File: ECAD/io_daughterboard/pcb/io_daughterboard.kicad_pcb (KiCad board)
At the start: 2 copper layers, 120 x 66 mm, 90 parts, among them CON1 BARREL_JACK, J1 XF2L-0625-1A, J2 FH12A-40S-0.5SH, P1 CONN_02X32, P10 Slave 5B, P11 Slave 1C, P12 Slave 3C, P13 Slave 4C, P14 Slave 5C, P15 Slave 1D, P16 Slave 3D, P17 Slave 4D, P18 Slave 5D, P19 MIDI, P2 CONN_02X32, P3 Slave 1A, P4 Slave 3A, P5 Slave 4A, P6 Slave 5A, P7 Slave 1B, P8 Slave 3B, P9 Slave 4B, SW1 Reset, SW2 User, U1 FAN5333BSX, U10 SN74LV1T34DCKR, U11 SN74LV1T34DCKR, U2 SPX3819M5-L-3-3, U3 74HC244, U4 74HC244, U5 74HC244, U6 STMPE811QTR, U7 74HC244, U8 74HC244, U9 74HC244

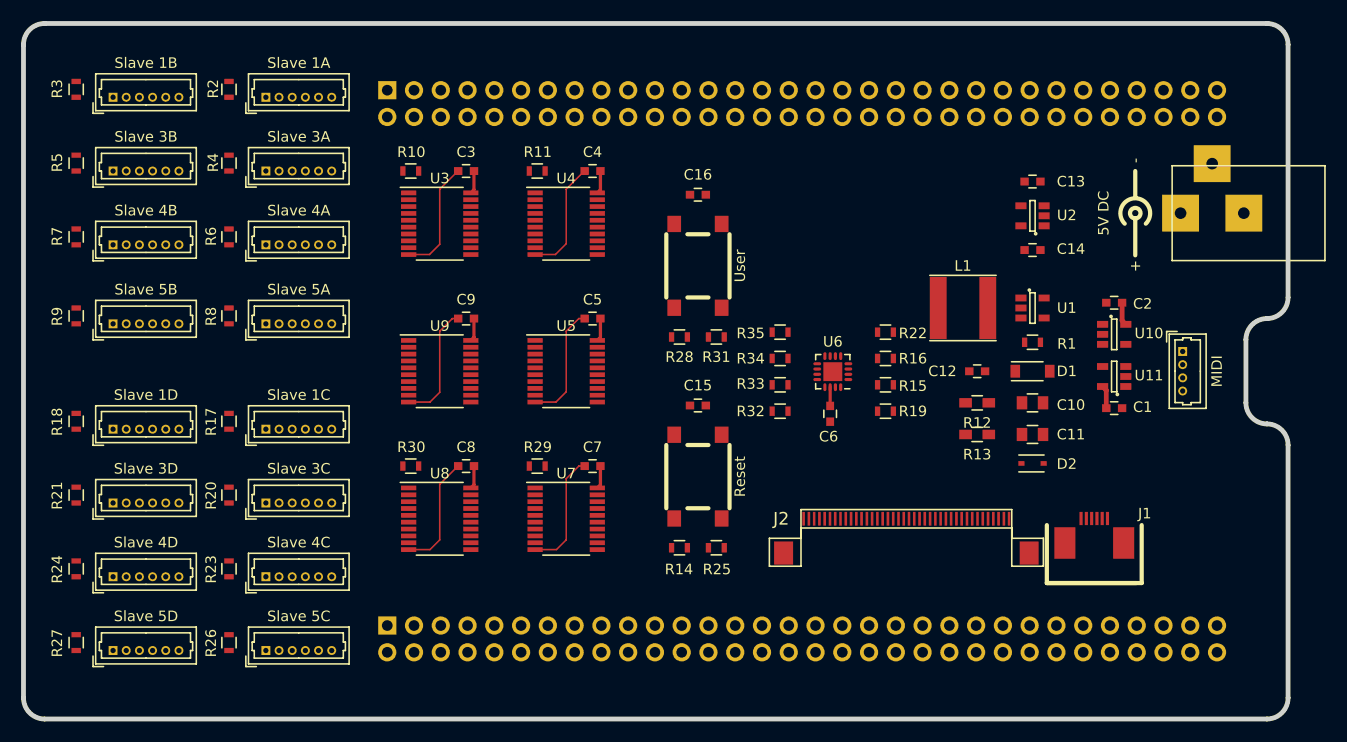
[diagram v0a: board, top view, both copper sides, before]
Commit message: Autorouted.
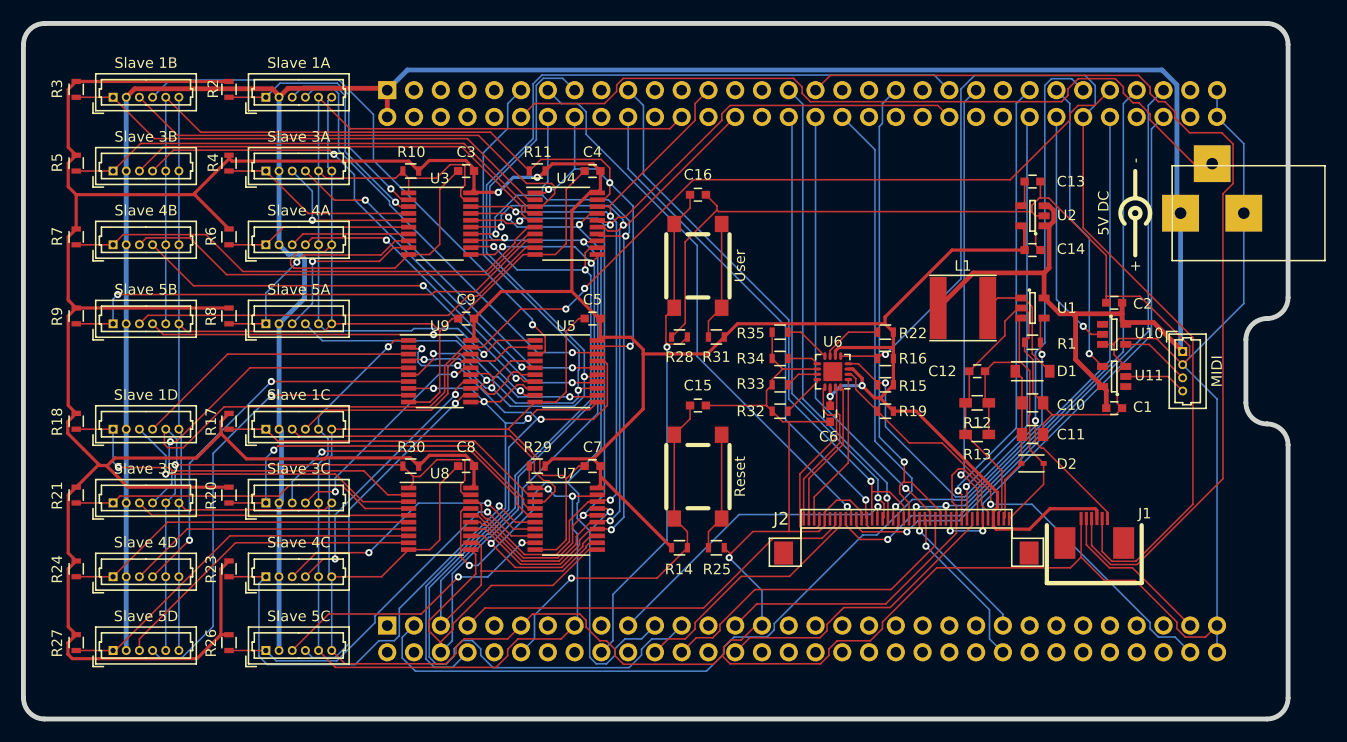
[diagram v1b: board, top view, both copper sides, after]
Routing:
- net GND: track 67.2 -> 632.6 mm, vias 0 -> 1
- net +3V3: track 15.0 -> 394.0 mm, vias 0 -> 4
- net +5V: track 4.39 -> 286.9 mm
- net /PC8: track 0.00 -> 163.3 mm, vias 0 -> 3
- net /I²C3_SDA: track 0.00 -> 105.2 mm, vias 0 -> 1
- net /PE3: track 0.00 -> 104.4 mm, vias 0 -> 3
- net /PC12: track 0.00 -> 104.2 mm, vias 0 -> 3
- net /PB7: track 0.00 -> 101.0 mm, vias 0 -> 1
- net /PC11: track 0.00 -> 97.6 mm, vias 0 -> 3
- net /CTOUCH_WAKE: track 0.00 -> 94.9 mm
- net /PA7: track 0.00 -> 92.4 mm, vias 0 -> 3
- net /PA5: track 0.00 -> 89.5 mm, vias 0 -> 4
- net /PF7: track 0.00 -> 87.7 mm, vias 0 -> 2
- net /LCD_PWM: track 0.00 -> 85.5 mm, vias 0 -> 1
- net /PC3: track 0.00 -> 82.6 mm, vias 0 -> 3
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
